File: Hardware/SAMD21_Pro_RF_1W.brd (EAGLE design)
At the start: 53.3 x 40.6 mm, 143 parts, among them J10 AVR_SPI_PROG_3X2TESTPOINTS, J12 JST, J13 U.FL, J14 RFM_DIO, J7 PTH, J9 External On/Off, U1 MCP73831, U2 ADJ3.3, U4 ATSAMD21G, U5 4MB Flash, U6 E19-915MS1W, U7 ADJ5, U8 TXB0108DQSR, U9 TXB0108DQSR, Y1 32.768kHz

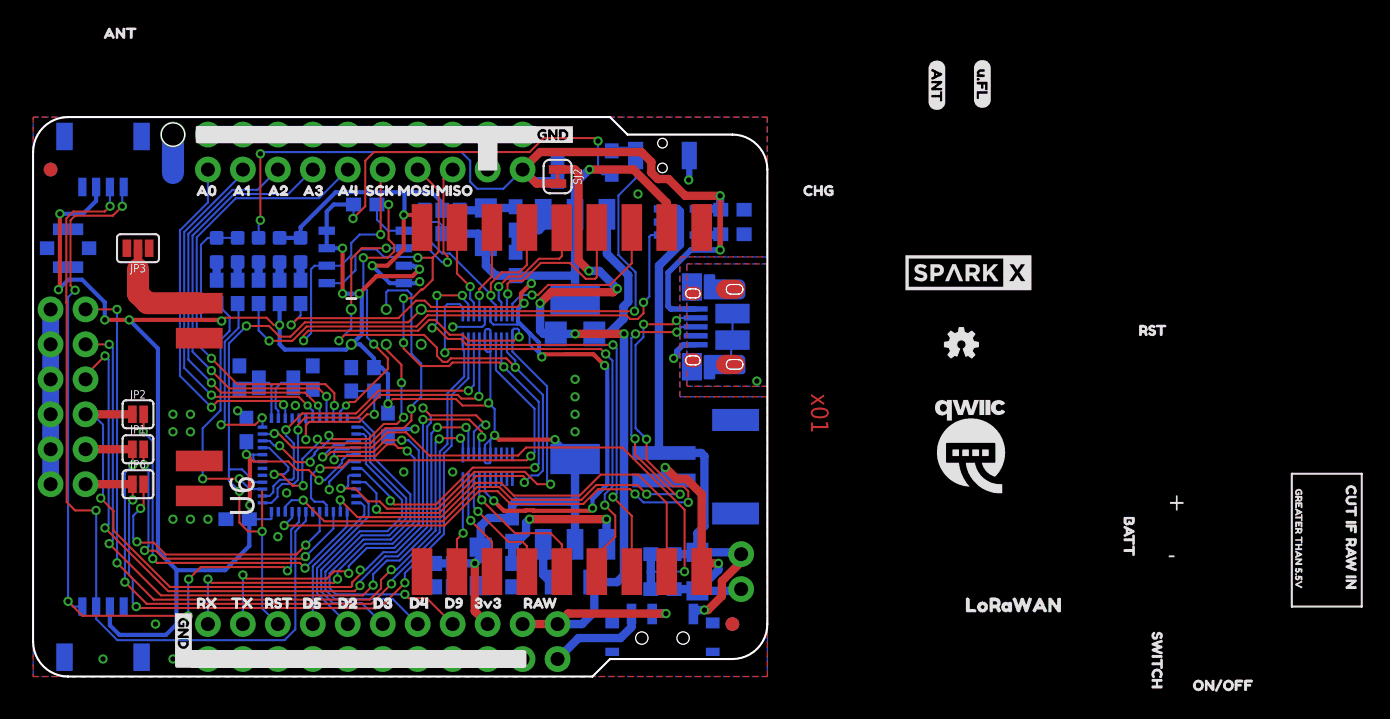
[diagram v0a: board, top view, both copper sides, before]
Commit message: Almost done
ToDo: Ask for guidance on antenna traces, double check on if the same chip is used (to know how to connect DIO pins), get board/schem review, order
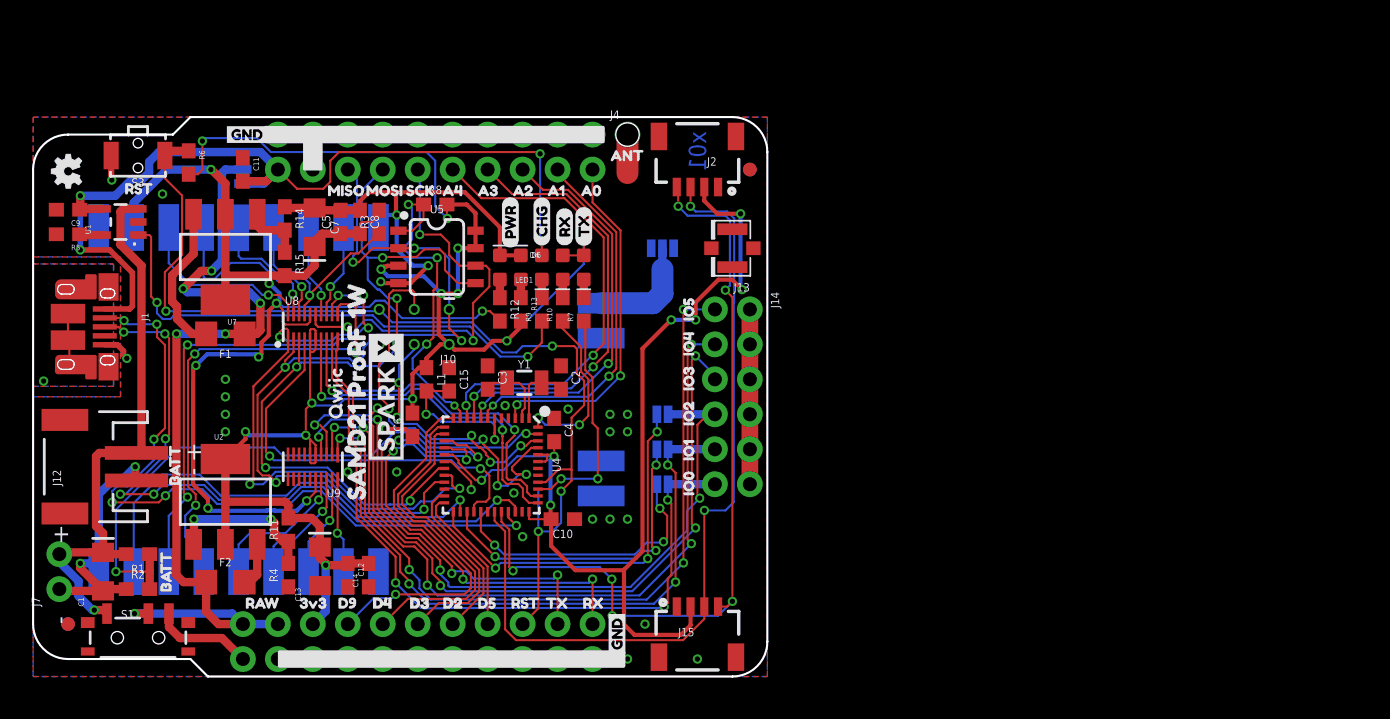
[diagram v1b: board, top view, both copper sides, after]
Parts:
- removed U$1: (no value), SAMD21:SAMD21_PRO_RF0
- removed U$14, U$40: (no value), buzzard_labels (25):CHG1
- removed U$27, U$37: (no value), buzzard_labels (25):SWITCH23
- added U$64, U$75: (no value), buzzard_labels:IO00
- added U$66, U$76: (no value), buzzard_labels:IO11
- added U$67, U$77: (no value), buzzard_labels:IO22
- added U$68, U$78: (no value), buzzard_labels:IO33
- added U$71, U$79: (no value), buzzard_labels:IO44
- added U$74, U$80: (no value), buzzard_labels:IO55
- added U$81: (no value), buzzard_labels:SAMD21_PRORF_1W5
- moved U$26 121.9 mm to (-34.3, -14.0), flipped to the top
- moved U$58 84.1 mm to (14.6, 36.8), flipped to the bottom, turned to 0 degrees
- moved FRAME2 81.3 mm to (-14.0, -12.7), flipped to the top
- moved U$59 80.8 mm to (14.1, 35.8), flipped to the bottom, turned to 0 degrees
- moved U$28 77.6 mm to (5.97, 35.4), flipped to the top
- moved U$39 73.2 mm to (10.4, 1.91), flipped to the bottom
- moved U$36 71.7 mm to (9.27, 38.7), flipped to the bottom
- moved U$29 70.1 mm to (9.65, 5.46), flipped to the top
- moved U$32 69.3 mm to (10.3, 13.2), turned to 90 degrees
- moved LOGO1 66.1 mm to (2.54, 36.7), flipped to the bottom, turned to 270 degrees
- moved U$61 66.1 mm to (2.54, 36.7), flipped to the top, turned to 90 degrees
- moved FD2 50.8 mm to (52.1, 36.8), flipped to the bottom
- moved FD4 50.8 mm to (52.1, 36.8), flipped to the top
- moved U6 50.8 mm to (1.27, 7.62), flipped to the bottom
- moved J7 49.5 mm to (1.91, 6.35), flipped to the top
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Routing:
- net 3.3V: track 212.6 -> 204.0 mm
- net 5V: track 104.2 -> 100.3 mm
- net TX_LED: track 18.6 -> 16.5 mm
- net GND: track 125.5 -> 127.1 mm
- net SCK: track 66.7 -> 65.4 mm
- net USB_VCC: track 66.2 -> 67.5 mm
- net D9: track 28.4 -> 27.5 mm
- net D3: track 22.2 -> 21.3 mm
- net D4: track 24.9 -> 24.0 mm
- net RX_LED: track 13.2 -> 12.5 mm
- net TXO: track 34.8 -> 34.1 mm
- net RXI: track 34.3 -> 33.6 mm
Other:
- outline, holes or cut-outs redrawn
